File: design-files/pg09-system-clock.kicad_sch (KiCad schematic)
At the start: 10 parts, among them J201 Clock Speed, U201 CD74ACT109, U202 CD74ACT163, U204 GAL22V10, X201 ACO-32.000MHz

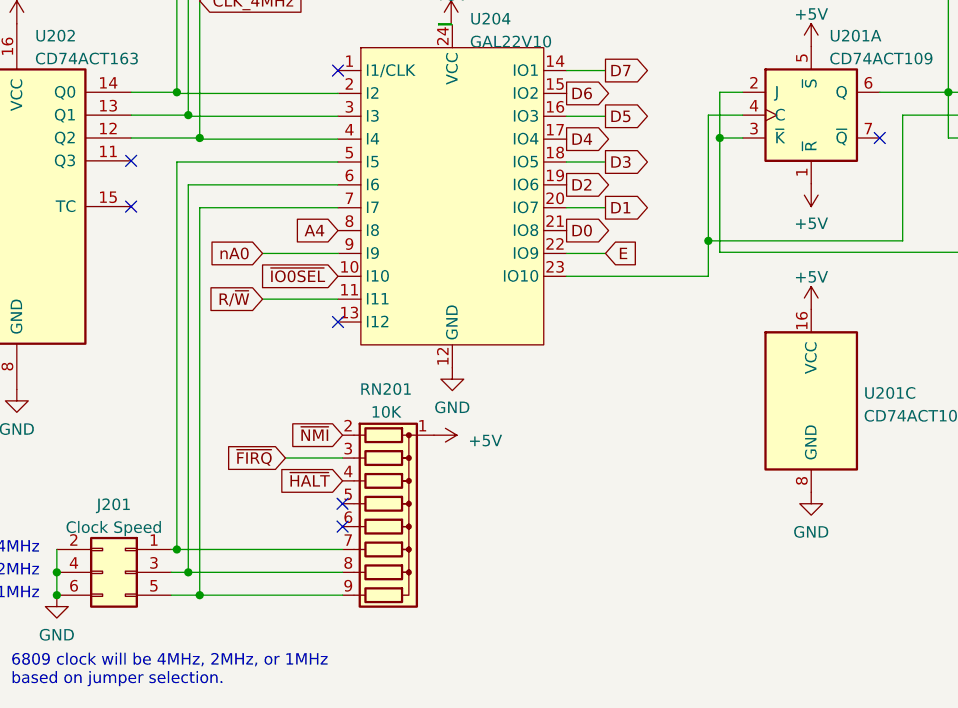
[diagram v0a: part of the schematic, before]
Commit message: Pull-up /RESET on RN201.
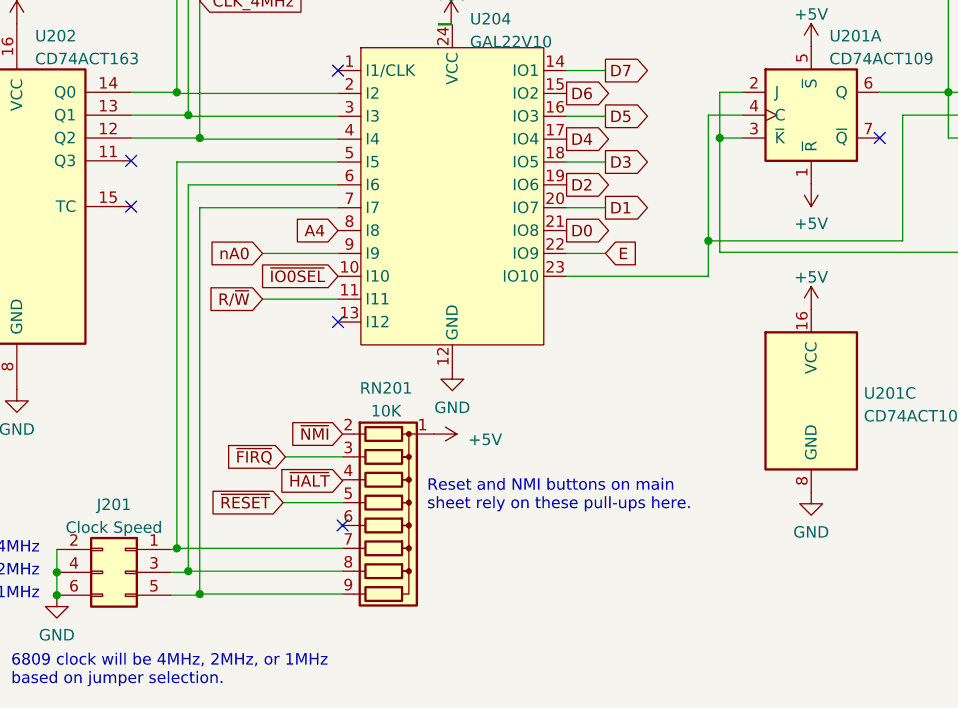
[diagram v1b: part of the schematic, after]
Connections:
- net ~{RESET}: now reaches RN201.5 (R4)
- no-connect marks 7 -> 6
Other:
- note added: "Reset and NMI buttons on main sheet rely on these pull-ups here."
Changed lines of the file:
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@@
   (junction (at 114.935 79.375) (diameter 0) (color 0 0 0 0)
   )
-  (junction (at 113.665 127.635) (diameter 0) (color 0 0 0 0)
+  (junction (at 114.935 130.048) (diameter 0) (color 0 0 0 0)
   )
   (junction (at 83.185 89.535) (diameter 0) (color 0 0 0 0)
@@
   (junction (at 116.205 81.915) (diameter 0) (color 0 0 0 0)
   )
-  (junction (at 114.935 130.175) (diameter 0) (color 0 0 0 0)
-  )
   (junction (at 229.235 113.03) (diameter 0) (color 0 0 0 0)
   )
@@
   (junction (at 229.235 107.95) (diameter 0) (color 0 0 0 0)
   )
-  (junction (at 116.205 132.715) (diameter 0) (color 0 0 0 0)
-  )
   (junction (at 100.33 132.715) (diameter 0) (color 0 0 0 0)
   )
@@
   (junction (at 208.915 113.03) (diameter 0) (color 0 0 0 0)
   )
+  (junction (at 113.665 127.508) (diameter 0) (color 0 0 0 0)
+  )
   (junction (at 113.665 76.835) (diameter 0) (color 0 0 0 0)
+  )
+  (junction (at 116.205 132.588) (diameter 0) (color 0 0 0 0)
   )
   (junction (at 83.185 81.915) (diameter 0) (color 0 0 0 0)
@@
   (no_connect (at 108.585 84.455))
   (no_connect (at 191.77 81.915))
-  (no_connect (at 132.08 125.095))
-  (no_connect (at 132.08 122.555))
+  (no_connect (at 132.08 124.968))
   (wire (pts (xy 113.03 130.175) (xy 114.935 130.175))
     (stroke (width 0) (type default))
@@
     (stroke (width 0) (type default))
   )
+  (wire (pts (xy 125.476 122.428) (xy 132.08 122.428))
+    (stroke (width 0) (type default))
+  )
   (wire (pts (xy 228.6 76.835) (xy 228.6 66.802))
     (stroke (width 0) (type default))
@@
     (stroke (width 0) (type default))
   )
-  (wire (pts (xy 125.73 117.475) (xy 132.08 117.475))
+  (wire (pts (xy 125.73 117.348) (xy 132.08 117.348))
     (stroke (width 0) (type default))
   )
@@
     (stroke (width 0) (type default))
   )
+  (wire (pts (xy 113.665 127.508) (xy 113.665 127.635))
+    (stroke (width 0) (type default))
+  )
   (wire (pts (xy 113.665 59.055) (xy 113.665 76.835))
     (stroke (width 0) (type default))
@@
     (stroke (width 0) (type default))
   )
-  (wire (pts (xy 114.935 130.175) (xy 132.08 130.175))
+  (wire (pts (xy 114.935 130.048) (xy 132.08 130.048))
     (stroke (width 0) (type default))
   )
@@
     (stroke (width 0) (type default))
   )
+  (wire (pts (xy 116.205 132.588) (xy 116.205 132.715))
+    (stroke (width 0) (type default))
+  )
   (wire (pts (xy 219.075 113.03) (xy 229.235 113.03))
     (stroke (width 0) (type default))
   )
-  (wire (pts (xy 116.205 89.662) (xy 116.205 132.715))
-    (stroke (width 0) (type default))
-  )
-  (wire (pts (xy 114.935 87.122) (xy 114.935 130.175))
+  (wire (pts (xy 116.205 89.662) (xy 116.205 132.588))
+    (stroke (width 0) (type default))
+  )
+  (wire (pts (xy 114.935 87.122) (xy 114.935 130.048))
     (stroke (width 0) (type default))
   )
@@
     (stroke (width 0) (type default))
   )
+  (wire (pts (xy 114.935 130.048) (xy 114.935 130.175))
+    (stroke (width 0) (type default))
+  )
   (wire (pts (xy 83.185 81.915) (xy 83.185 84.455))
     (stroke (width 0) (type default))
@@
     (stroke (width 0) (type default))
   )
-  (wire (pts (xy 113.665 84.582) (xy 113.665 127.635))
+  (wire (pts (xy 113.665 84.582) (xy 113.665 127.508))
+    (stroke (width 0) (type default))
+  )
+  (wire (pts (xy 132.08 119.888) (xy 132.08 120.015))
     (stroke (width 0) (type default))
   )
@@
     (stroke (width 0) (type default))
   )
-  (wire (pts (xy 113.665 127.635) (xy 132.08 127.635))
+  (wire (pts (xy 113.665 127.508) (xy 132.08 127.508))
     (stroke (width 0) (type default))
   )
@@
     (stroke (width 0) (type default))
   )
-  (wire (pts (xy 116.205 132.715) (xy 132.08 132.715))
+  (wire (pts (xy 116.205 132.588) (xy 132.08 132.588))
     (stroke (width 0) (type default))
   )
@@
   (text "4MHz" (at 98.425 128.27 0)
     (effects (font (size 1.27 1.27)) (justify right bottom))
+  )
+  (text "Reset and NMI buttons on main\nsheet rely on these pull-ups here."
+    (at 141.478 123.444 0)
+    (effects (font (size 1.27 1.27)) (justify left bottom))
   )
   (text "2MHz" (at 98.425 130.81 0)
@@
     )
   )
+  (global_label "~{RESET}" (shape input) (at 125.476 122.428 180) (fields_autoplaced)
+    (effects (font (size 1.27 1.27)) (justify right))
+    (property "Intersheetrefs" "${INTERSHEET_REFS}" (at 116.8251 122.428 0)
+      (effects (font (size 1.27 1.27)) (justify right) hide)
+    )
+  )
   (global_label "D4" (shape output) (at 156.972 82.042 0) (fields_autoplaced)
     (effects (font (size 1.27 1.27)) (justify left))
@@
     )
   )
-  (global_label "~{FIRQ}" (shape input) (at 125.73 117.475 180) (fields_autoplaced)
+  (global_label "~{FIRQ}" (shape input) (at 125.73 117.348 180) (fields_autoplaced)
     (effects (font (size 1.27 1.27)) (justify right))
-    (property "Intersheetrefs" "${INTERSHEET_REFS}" (at 118.5303 117.475 0)
+    (property "Intersheetrefs" "${INTERSHEET_REFS}" (at 118.5303 117.348 0)
       (effects (font (size 1.27 1.27)) (justify right) hide)
     )
@@
     )
   )
-  (global_label "~{NMI}" (shape input) (at 132.08 114.935 180) (fields_autoplaced)
+  (global_label "~{NMI}" (shape input) (at 132.08 114.808 180) (fields_autoplaced)
     (effects (font (size 1.27 1.27)) (justify right))
-    (property "Intersheetrefs" "${INTERSHEET_REFS}" (at 125.7875 114.935 0)
+    (property "Intersheetrefs" "${INTERSHEET_REFS}" (at 125.7875 114.808 0)
       (effects (font (size 1.27 1.27)) (justify right) hide)
     )
@@
     )
   )
-  (symbol (lib_id "Device:R_Network08") (at 137.16 125.095 270) (unit 1)
-    (in_bom yes) (on_board yes) (dnp no) (fields_autoplaced)
-    (property "Reference" "RN201" (at 136.906 109.855 90)
-      (effects (font (size 1.27 1.27)))
-    )
-    (property "Value" "10K" (at 136.906 112.395 90)
-      (effects (font (size 1.27 1.27)))
-    )
-    (property "Footprint" "Resistor_THT:R_Array_SIP9" (at 137.16 137.16 90)
-      (effects (font (size 1.27 1.27)) hide)
-    )
-    (property "Datasheet" "http://www.vishay.com/docs/31509/csc.pdf" (at 137.16 125.095 0)
+  (symbol (lib_id "Device:R_Network08") (at 137.16 124.968 270) (unit 1)
+    (in_bom yes) (on_board yes) (dnp no) (fields_autoplaced)
+    (property "Reference" "RN201" (at 136.906 109.728 90)
+      (effects (font (size 1.27 1.27)))
+    )
+    (property "Value" "10K" (at 136.906 112.268 90)
+      (effects (font (size 1.27 1.27)))
+    )
+    (property "Footprint" "Resistor_THT:R_Array_SIP9" (at 137.16 137.033 90)
+      (effects (font (size 1.27 1.27)) hide)
+    )
+    (property "Datasheet" "http://www.vishay.com/docs/31509/csc.pdf" (at 137.16 124.968 0)
       (effects (font (size 1.27 1.27)) hide)
     )
@@
     )
   )
-  (symbol (lib_id "power:+5V") (at 142.24 114.935 270) (unit 1)
-    (in_bom yes) (on_board yes) (dnp no) (fields_autoplaced)
-    (property "Reference" "#PWR0221" (at 138.43 114.935 0)
-      (effects (font (size 1.27 1.27)) hide)
-    )
-    (property "Value" "+5V" (at 146.05 115.57 90)
-      (effects (font (size 1.27 1.27)) (justify left))
-    )
-    (property "Footprint" "" (at 142.24 114.935 0)
-      (effects (font (size 1.27 1.27)) hide)
-    )
-    (property "Datasheet" "" (at 142.24 114.935 0)
-      (effects (font (size 1.27 1.27)) hide)
-    )
+  (symbol (lib_id "power:+5V") (at 142.24 114.808 270) (unit 1)
+    (in_bom yes) (on_board yes) (dnp no) (fields_autoplaced)
+    (property "Reference" "#PWR0221" (at 138.43 114.808 0)
+      (effects (font (size 1.27 1.27)) hide)
+    )
+    (property "Value" "+5V" (at 146.05 115.443 90)
+      (effects (font (size 1.27 1.27)) (justify left))
+    )
+    (property "Footprint" "" (at 142.24 114.808 0)
+      (effects (font (size 1.27 1.27)) hide)
+    )
+    (property "Datasheet" "" (at 142.24 114.808 0)
+      (effects (font (size 1.27 1.27)) hide)
+    )
